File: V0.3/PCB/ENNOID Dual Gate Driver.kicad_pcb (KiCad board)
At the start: 2 copper layers, 60 x 98 mm, 142 parts, among them J1 Conn_02x08_Odd_Even, J10 Mounting Hole 2, J11 Mounting Hole 3, J2 Current, J3 TEMP, J4 PHASE, J5 Collector, J6 Gate_H, J7 G_L, J8 E, J9 Mounting hole 1, Q3 MJD3055T4G, Q4 MJD2955T4G, Q5 MJD3055T4G, Q6 MJD2955T4G, U1 MC7805, U2 MGJ2, U3 MGJ2, U4 ISO5852SDWR, U5 ISO5852SDWR, U8 AMC1301

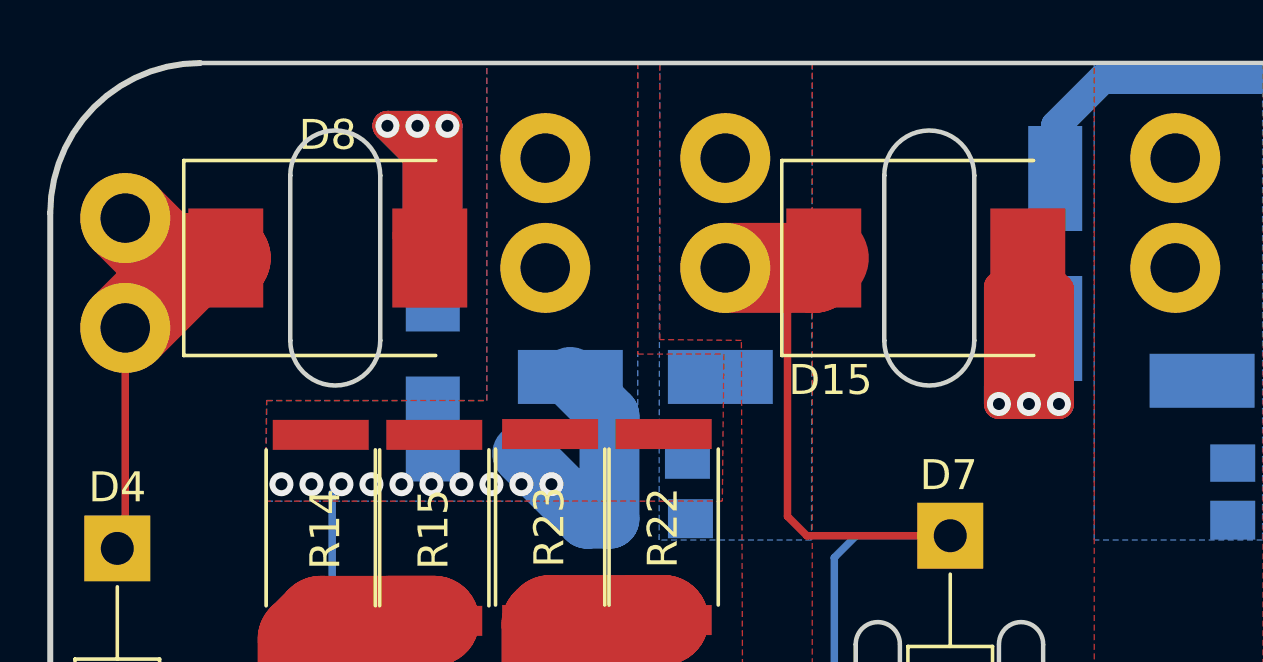
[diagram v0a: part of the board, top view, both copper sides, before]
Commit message: Maintenance update
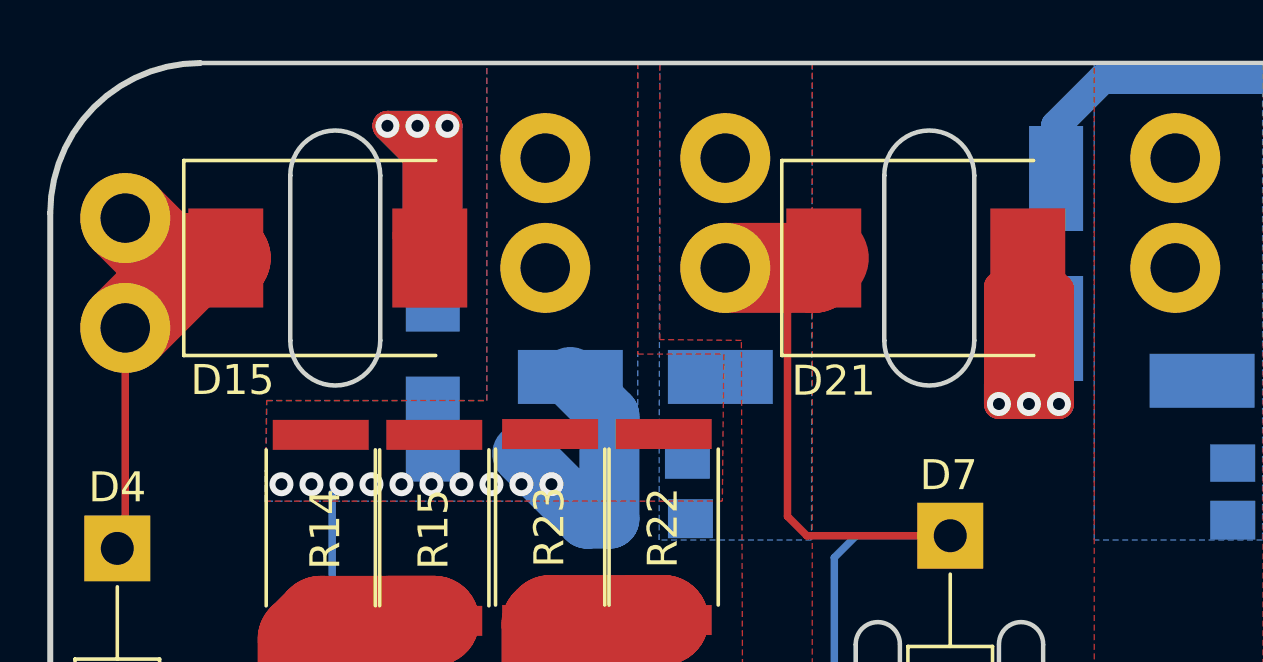
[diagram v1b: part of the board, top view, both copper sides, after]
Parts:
- D21: value es2j-ltp -> smcj440ca; footprint Diodes_SMD:D_SMA_Handsoldering -> Diodes_SMD:D_SMC; moved to F.Cu
- D8: value smcj440ca -> es2j-ltp; footprint Diodes_SMD:D_SMC -> Diodes_SMD:D_SMA_Handsoldering; moved to B.Cu
- moved D8 24.3 mm to (33.5, 6.35), turned to 270 degrees
- moved D5 21.0 mm to (12.8, 9.70), turned to 90 degrees
- moved D15 19.9 mm to (9.25, 6.50)
- moved D21 16.7 mm to (29.2, 6.50), turned to 0 degrees
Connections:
- D15 pad 1: PHASE -> /GD_HIGH/C
- D21 pad 1: /GD_HIGH/G -> PHASE
- D5 pad 1: /GD_LOW/G -> /GD_HIGH/G
- D8 pad 1: /GD_HIGH/C -> /GD_LOW/G
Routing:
- net Net-(D21-Pad2): track 35.8 -> 28.3 mm
- net Net-(D15-Pad2): track 28.3 -> 35.8 mm
